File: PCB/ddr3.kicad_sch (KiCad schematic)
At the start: 35 parts, among them U11 MT41J128M16JT-125:K

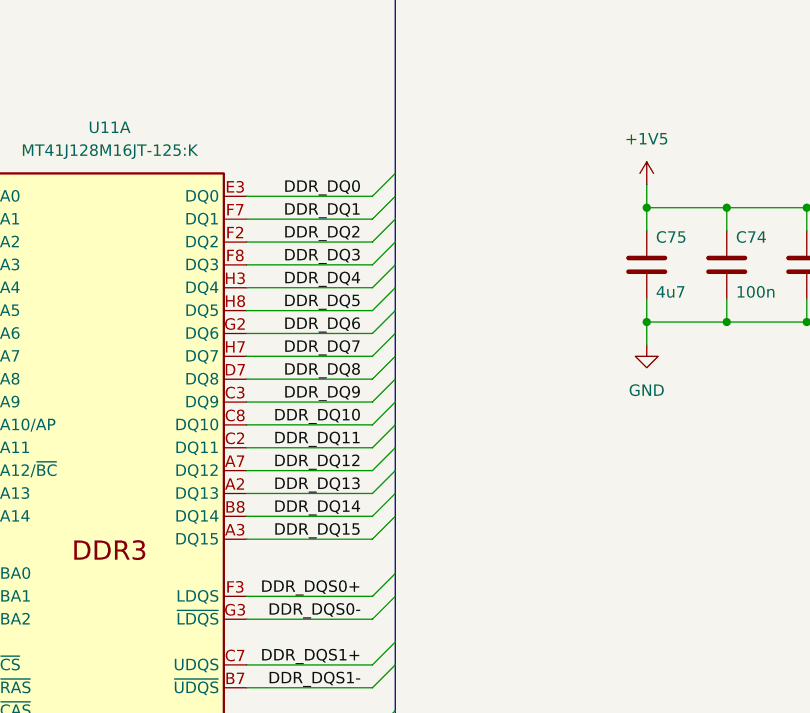
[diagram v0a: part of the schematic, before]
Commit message: properly matching all the signals
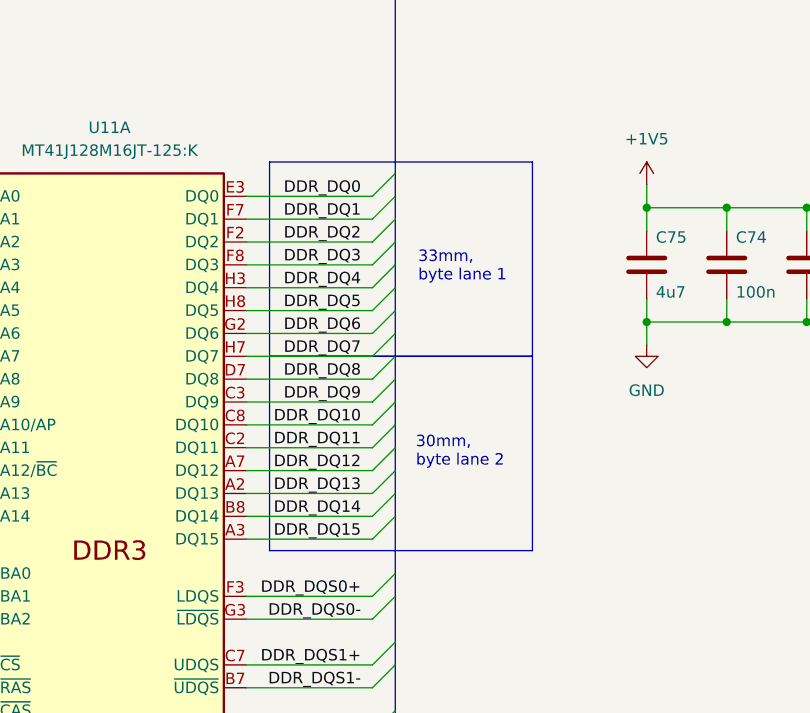
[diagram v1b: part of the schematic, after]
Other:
- note added: "30mm, byte lane 2"
- note added: "33mm, byte lane 1"
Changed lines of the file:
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@@
 	(generator_version "10.0")
 	(paper "A3")
+	(rectangle
+		(start 134.62 134.62)
+		(end 163.83 156.21)
+		(stroke
+			(width 0)
+			(type default)
+		)
+		(fill
+			(type none)
+		)
+	)
+	(rectangle
+		(start 134.62 113.03)
+		(end 163.83 134.62)
+		(stroke
+			(width 0)
+			(type default)
+		)
+		(fill
+			(type none)
+		)
+	)
 	(text "MT41J128M16JT-125:K\n16 Bit data width\n8 Bank machines\nNormal ordering"
 		(exclude_from_sim no)
@@
 		)
 	)
+	(text "33mm, \nbyte lane 1\n"
+		(exclude_from_sim no)
+		(at 151.13 124.714 0)
+		(effects
+			(font
+				(size 1.27 1.27)
+			)
+			(justify left)
+		)
+	)
 	(text "Shunt termination because\nCLK doesn't have ODT :("
 		(exclude_from_sim no)
@@
 		)
 	)
+	(text "30mm, \nbyte lane 2\n"
+		(exclude_from_sim no)
+		(at 150.876 145.288 0)
+		(effects
+			(font
+				(size 1.27 1.27)
+			)
+			(justify left)
+		)
+	)
